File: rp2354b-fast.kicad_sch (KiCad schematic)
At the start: 29 parts, among them J2 Conn_ARM_SWD_TagConnect_TC203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, SW1 SW_Push, SW2 SW_Push, U1 RP2354B, U4 BMP581, Y1 12MHz

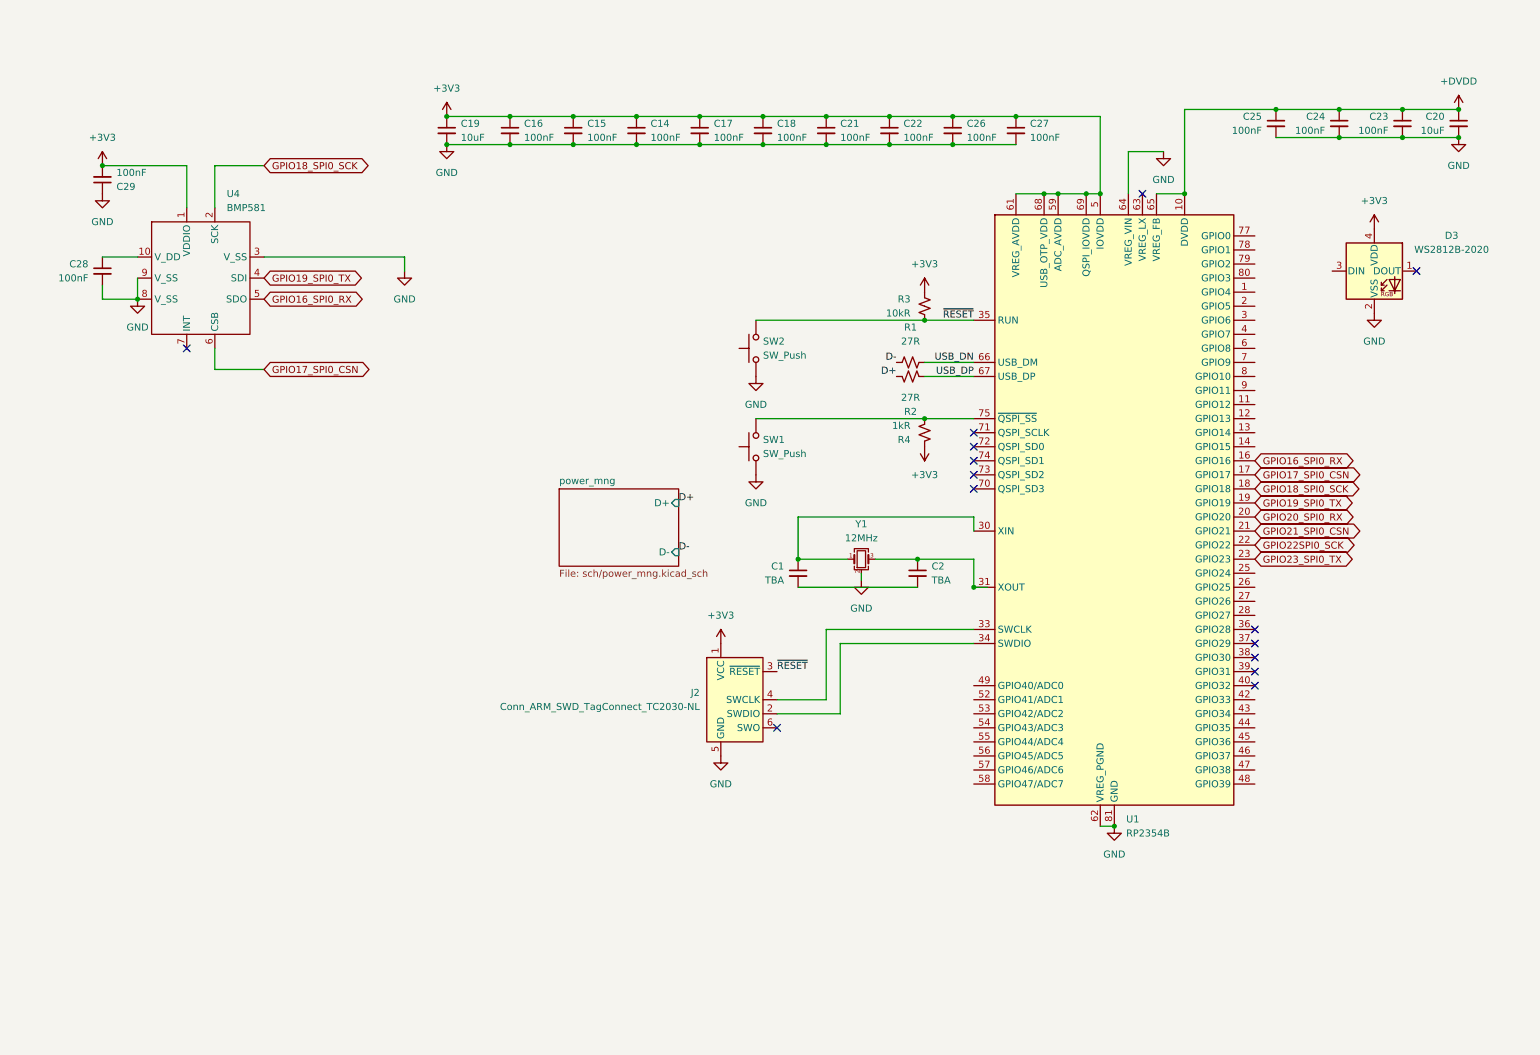
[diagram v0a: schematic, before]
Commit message: hv16v
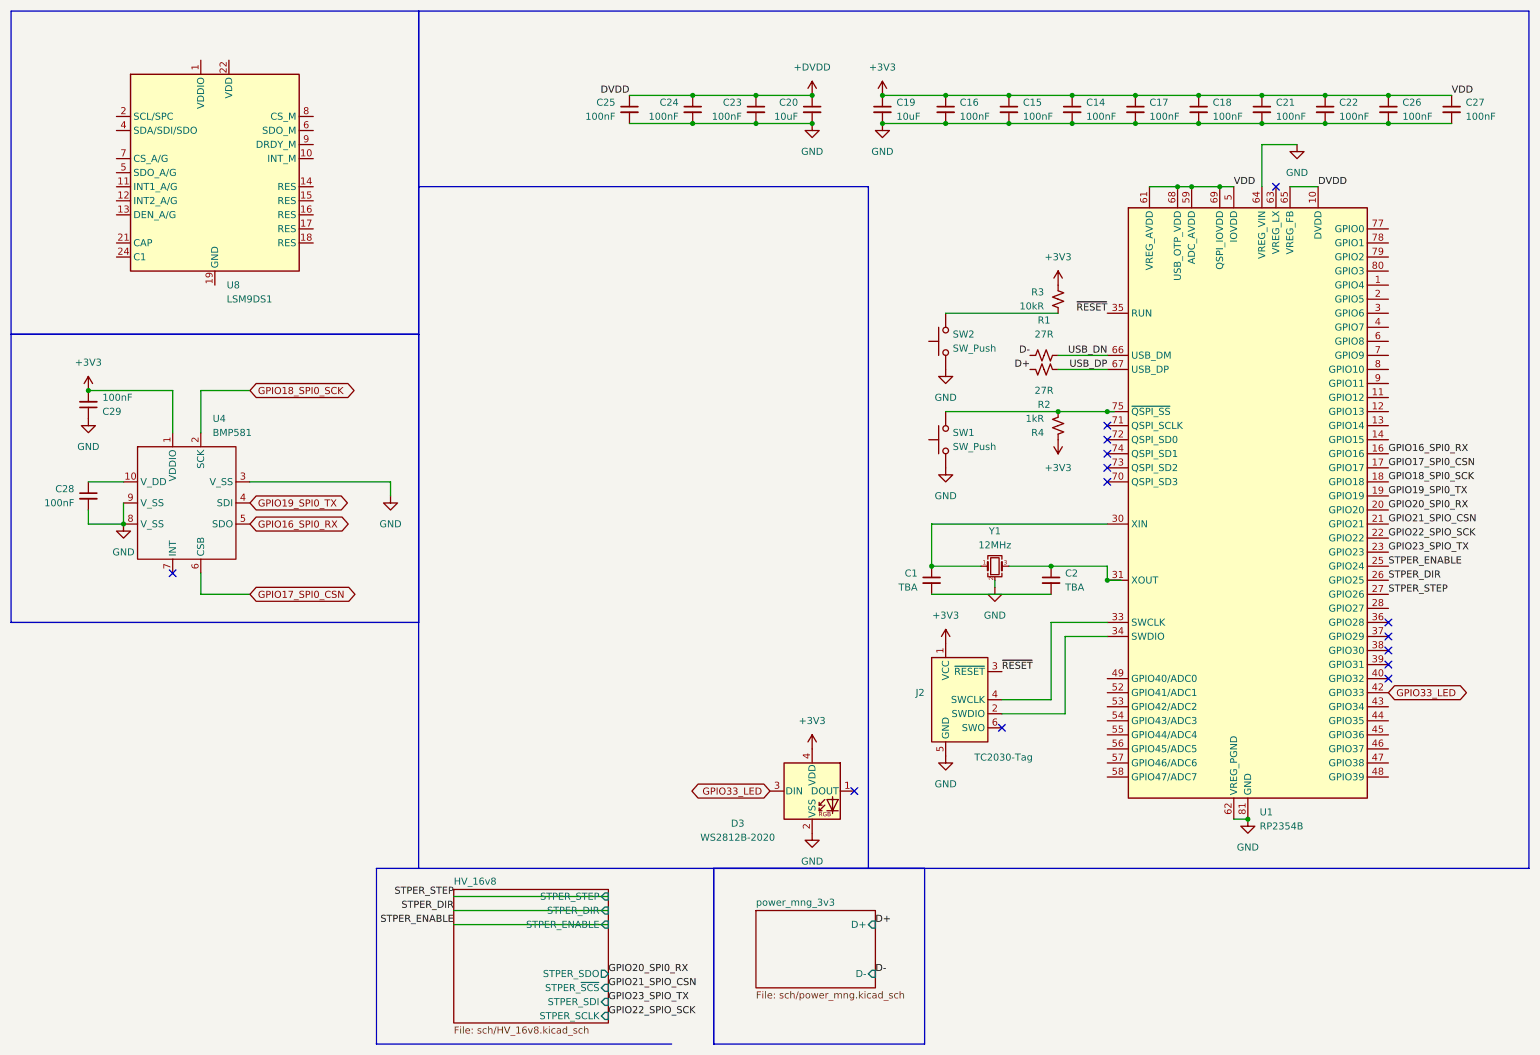
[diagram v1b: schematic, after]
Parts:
- added U8: LSM9DS1, Package_LGA:LGA-24L_3x3.5mm_P0.43mm, symbol Sensor_Motion:LSM9DS1
- J2: value Conn_ARM_SWD_TagConnect_TC2030-NL -> TC2030-Tag
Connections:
- net ~{RESET}: no longer R3.2, SW2.2
- net GPIO33_LED: now reaches D3.3 (DIN)
- net GPIO33_LED: now also U1.42 (GPIO33)
- net STPER_ENABLE: now reaches U1.25 (GPIO24)
- net STPER_DIR: now reaches U1.26 (GPIO25)
- net STPER_STEP: now reaches U1.27 (GPIO26)
- net GPIO21_SPI0_CSN renamed GPIO21_SPIO_CSN
- net GPIO22SPI0_SCK renamed GPIO22_SPIO_SCK
- net GPIO23_SPI0_TX renamed GPIO23_SPIO_TX
- new net: R3.2, SW2.2
- new net: U8.1 (VDDIO), U8.3 (VDDIO)
- new net: U8.19 (GND), U8.20 (GND)
- new net: U8.22 (VDD), U8.23 (VDD)
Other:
- sheet power_mng renamed power_mng_3v3
- added sheet HV_16v8 (sch/HV_16v8.kicad_sch)
- moved on the sheet: C1, C14, C15, C16, C17, C18, C19, C2, C20, C21, C22, C23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
